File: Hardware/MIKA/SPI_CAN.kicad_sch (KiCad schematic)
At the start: 35 parts, among them J10 CarCAN_Debug, J11 TelemCAN_Debug, J6 TelemCAN_Conn1, J7 CarCAN_Conn1, J8 CarCAN_Conn2, J9 TelemCAN_Conn2, U4 TCAN4551RGYRQ1, U5 TCAN4551RGYRQ1, Y1 7M40000005, Y2 Crystal_GND24

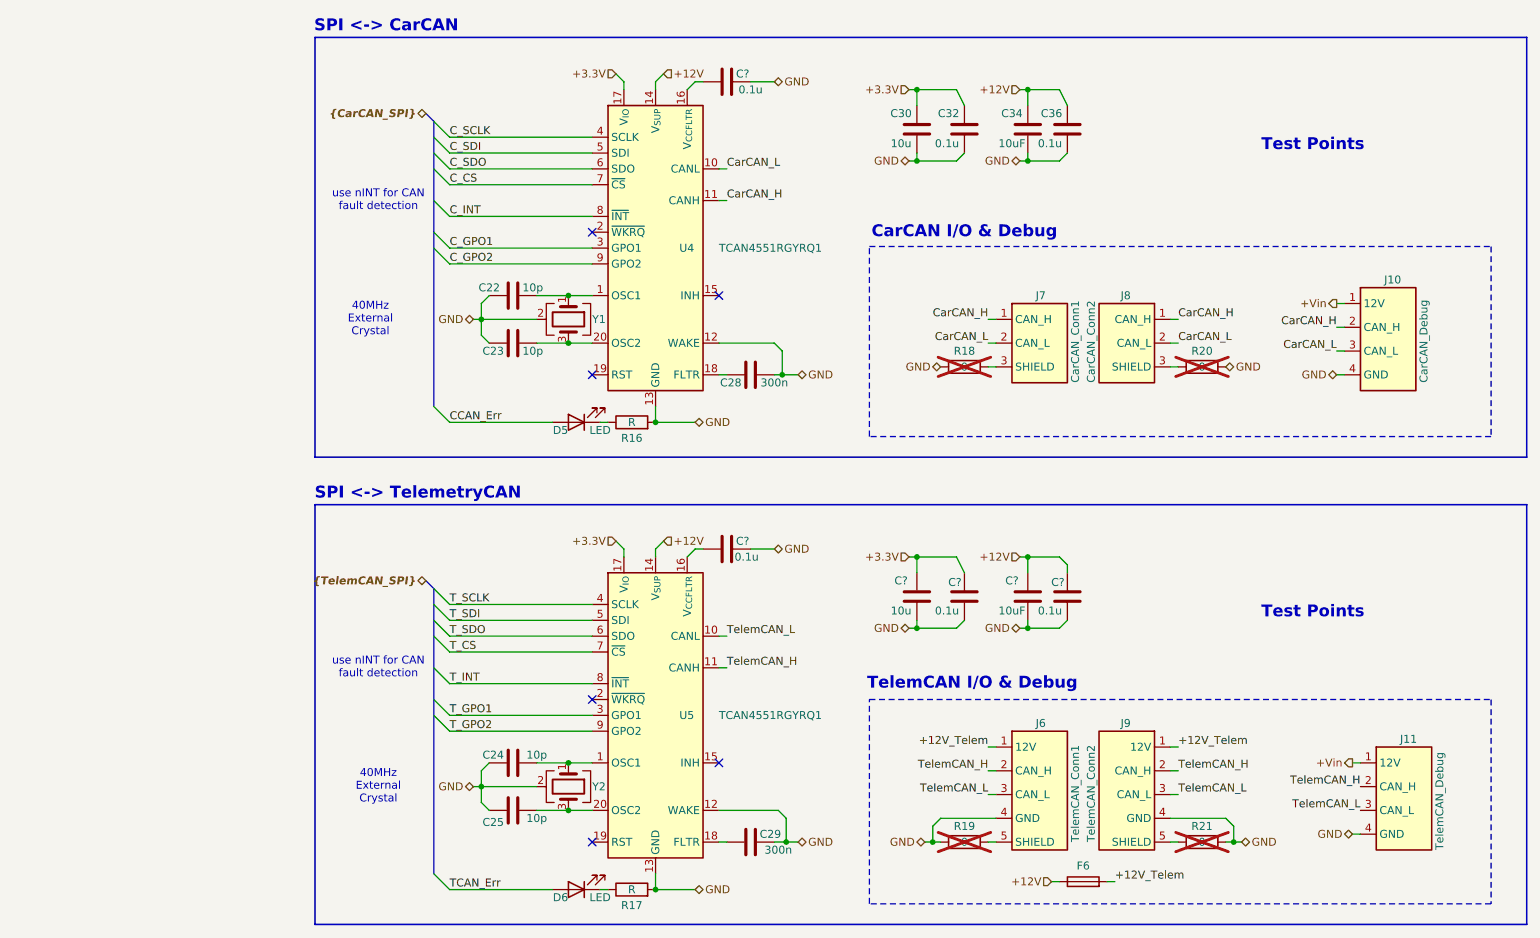
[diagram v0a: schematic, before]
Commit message: bahasdf;ladjsfhadf boooooooooooshksa
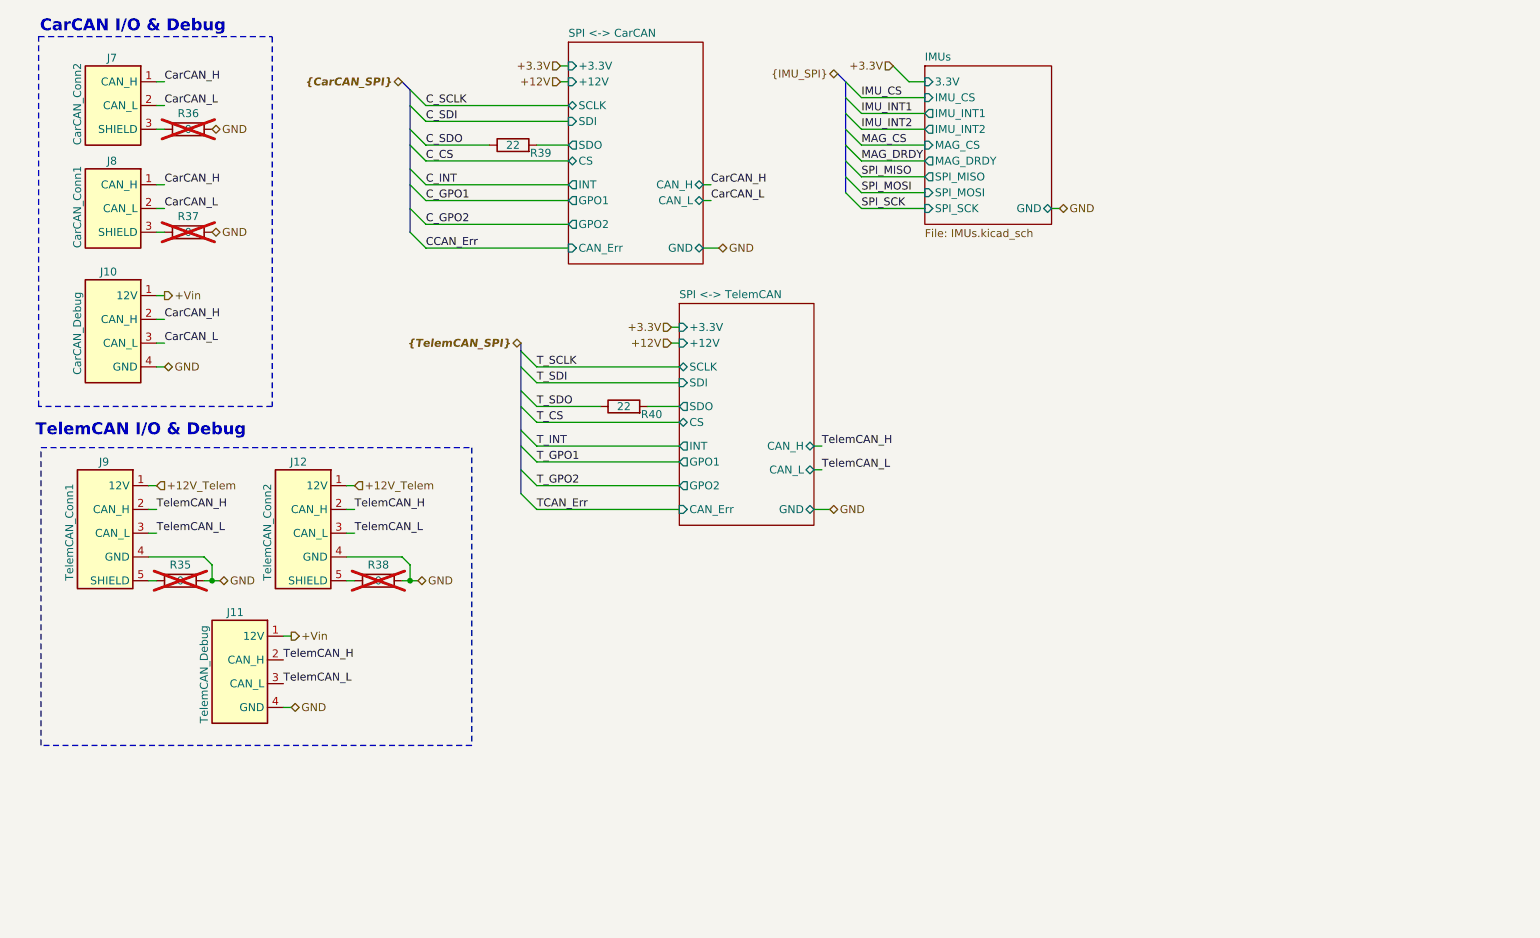
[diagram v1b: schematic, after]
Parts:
- removed C22, C23, C24, C25: 10p, symbol Device:C
- removed C28, C29: 300n, symbol Device:C
- removed C30, C?: 10u, symbol Device:C
- removed C32, C36, C? (x4): 0.1u, symbol Device:C
- removed C34, C?: 10uF, symbol Device:C
- removed D5, D6: LED, symbol Device:LED
- removed F6: Fuse, symbol Device:Fuse
- removed R16, R17: R, symbol Device:R
- removed U4, U5: TCAN4551RGYRQ1, Package_DFN_QFN:Texas_RGY_R-PVQFN-N20_EP2.05x3.05mm, symbol Interface_CAN_LIN:TCAN4551RGYRQ1
- removed Y1: 7M40000005, symbol Device:Crystal_GND24
- removed Y2: Crystal_GND24, symbol Device:Crystal_GND24
- added R39, R40: 22, symbol Device:R
- renumbered J9 to J12, J8 to J7, J7 to J8, J6 to J9, R19 to R35, R20 to R36, R18 to R37, R21 to R38
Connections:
- net C_SDO: now also R39.1
- net T_SDO: now also R40.1
- new net SPI <-> CarCAN/SDO: R39.2
- new net SPI <-> TelemCAN/SDO: R40.2
- no-connect marks 6 -> 0
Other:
- added sheet IMUs (IMUs.kicad_sch)
- added sheet SPI <-> CarCAN (spi_2_can.kicad_sch)
- added sheet SPI <-> TelemCAN (spi_2_can.kicad_sch)
- note removed: "40MHz External Crystal"
- note removed: "SPI <-> CarCAN"
- note removed: "SPI <-> TelemetryCAN"
- note removed: "Test Points"
- note removed: "use nINT for CAN fault detection"
- moved on the sheet: J10, J11, J12, J7, J8, J9, R35, R36, R37, R38
